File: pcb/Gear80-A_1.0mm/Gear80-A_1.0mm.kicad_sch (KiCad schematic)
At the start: 249 parts, among them J2 Conn_01x10_Pin, J3 Conn_01x04, J3 Conn_01x10_Pin, J4 Conn_01x10_Pin, J5 Conn_01x10_Pin, J6 Conn_01x10_Pin, J7 Conn_01x10_Pin, U1 XC6206P332MR, U3 W25Q128JVSIQ, U4 RP2040, Y1 X322512MSB4SI

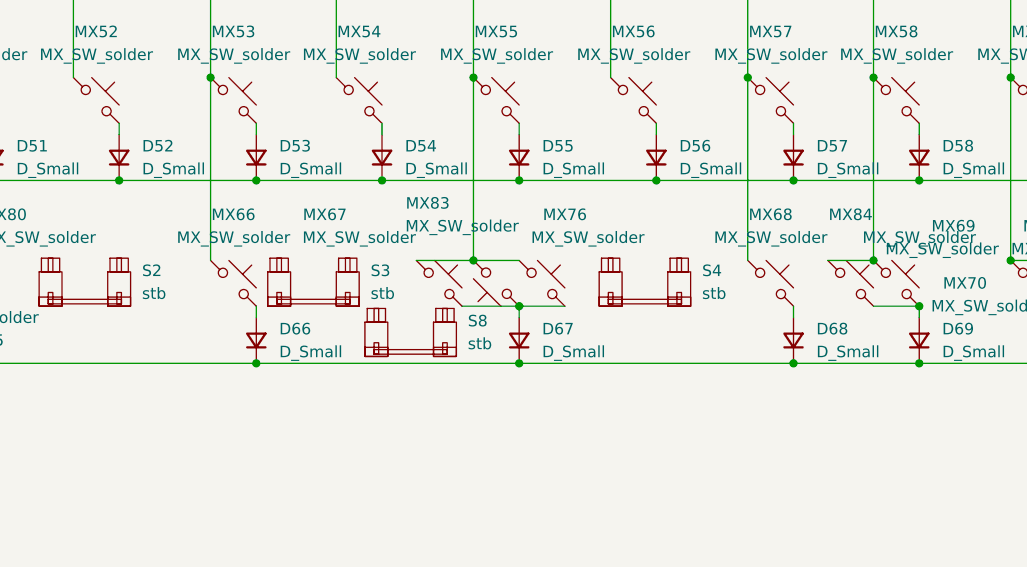
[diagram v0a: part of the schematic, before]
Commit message: Add files via upload
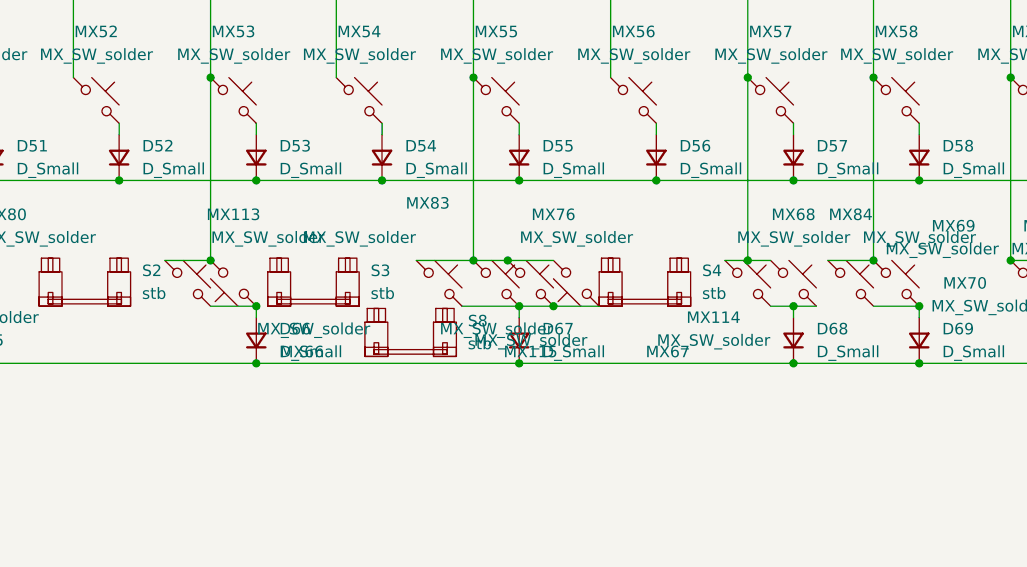
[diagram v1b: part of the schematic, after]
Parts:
- added MX113, MX114, MX115: MX_SW_solder, PCM_marbastlib-mx:SW_MX_1u, symbol PCM_marbastlib-mx:MX_SW_HS
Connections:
- net COL5: now also MX66.2, MX113.1; no longer MX66.1
- net COL7: now also MX67.1, MX115.2; no longer MX67.2
- net COL9: now also MX114.1
- net at D66.2 (A): now also MX66.1, MX113.2; no longer MX66.2
- net at D67.2 (A), MX76.2, MX83.2: now also MX67.2, MX115.1; no longer MX67.1
- net at D68.2 (A), MX68.2: now also MX114.2
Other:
- moved on the sheet: MX66, MX67, MX68, MX76
